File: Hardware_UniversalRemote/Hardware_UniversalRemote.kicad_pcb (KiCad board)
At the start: 2 copper layers, 140 x 140 mm, 58 parts, among them J1 USB_B_Micro, Q1 S8050, Q2 BSS138, Q3 S8050, Q4 S8050, Q5 S8050, Q6 S8050, Q7 S8050, SW1 SW_Push, SW2 SW_Push, SW3 SW_Push, U1 ESP32-WROOM-32U, U2 LM1117T-3.3, U3 HS0038B, U4 CH340C

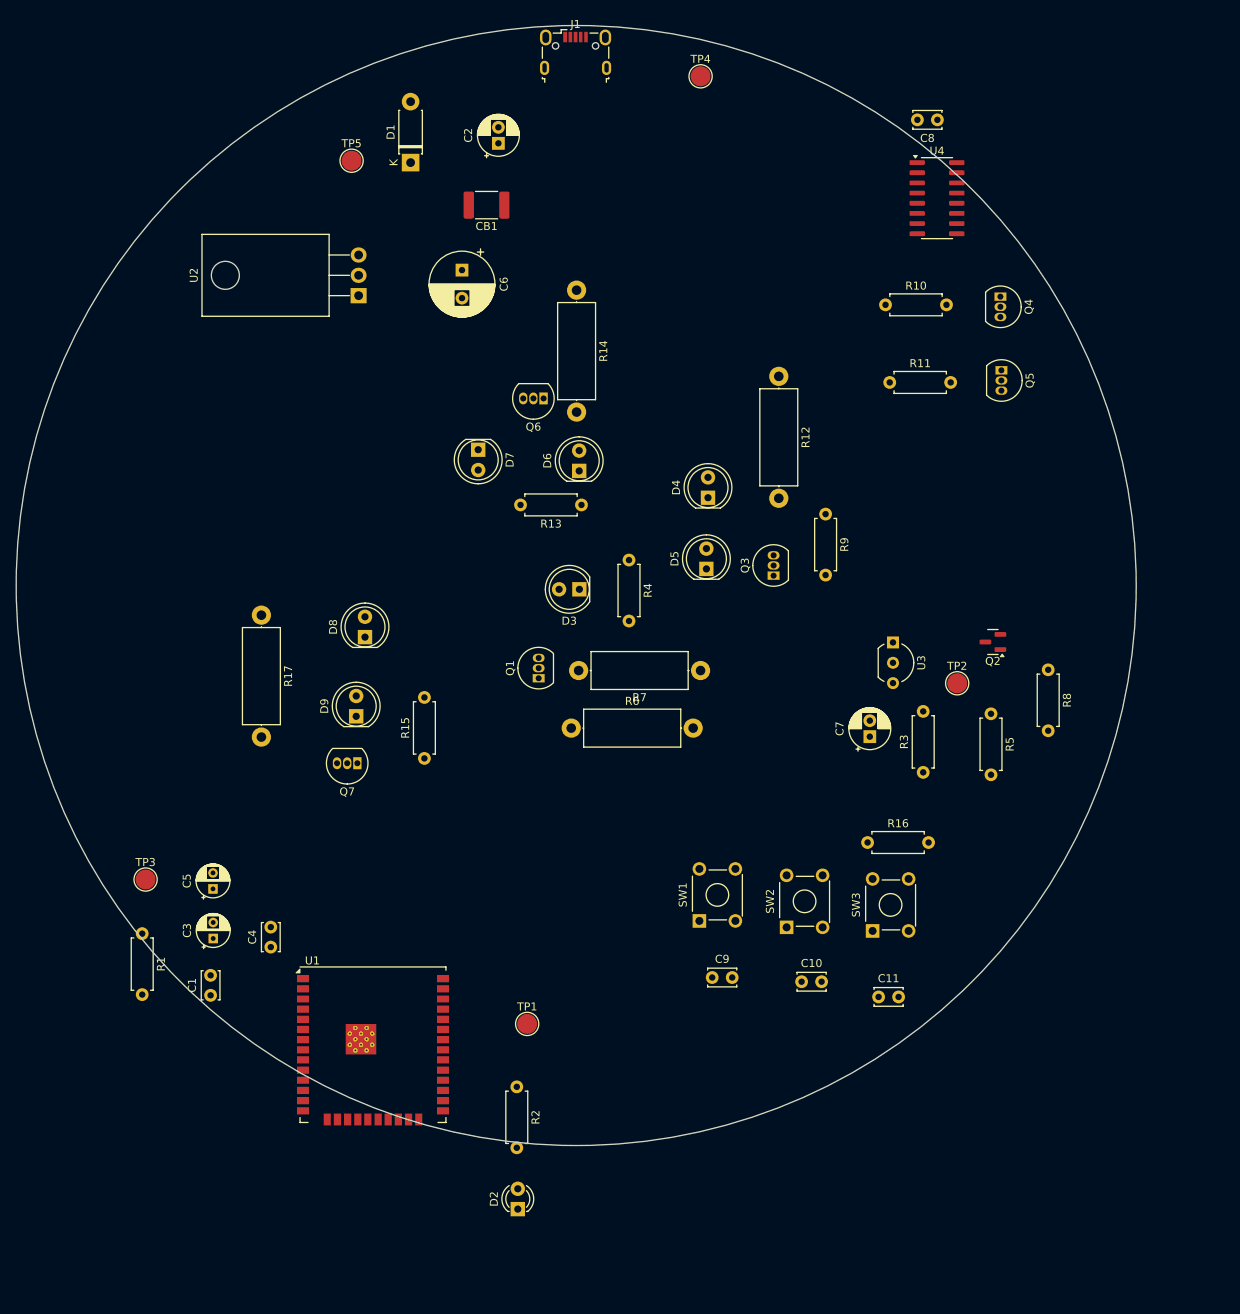
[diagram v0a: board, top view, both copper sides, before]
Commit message: add first pcb layout version
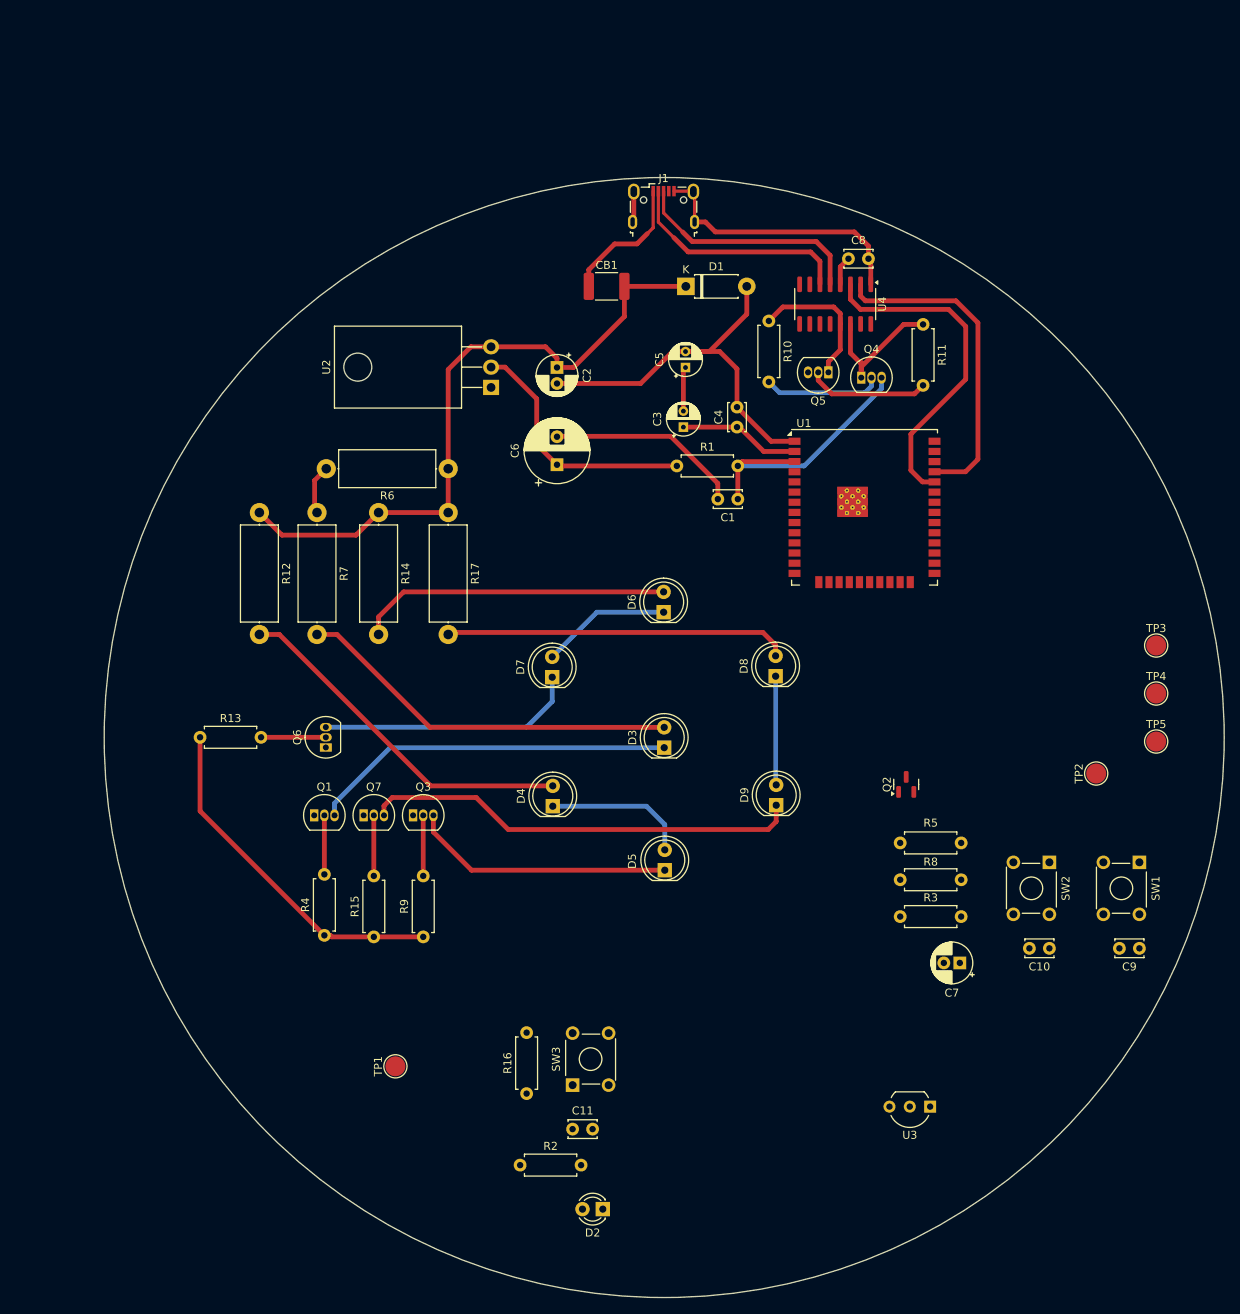
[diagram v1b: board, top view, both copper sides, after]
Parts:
- moved TP3 129.7 mm to (172.5, 107.5)
- moved TP5 124.0 mm to (172.5, 119.5)
- moved TP4 95.9 mm to (172.5, 113.5)
- moved U1 91.0 mm to (136.0, 90.2)
- moved C1 90.5 mm to (120.2, 89.2), turned to 180 degrees
- moved R1 88.8 mm to (112.6, 85.0), turned to 0 degrees
- moved C5 88.0 mm to (113.7, 72.8)
- moved C4 87.3 mm to (120.1, 80.2)
- moved C3 86.8 mm to (113.4, 80.2)
- moved R9 73.0 mm to (80.9, 143.9), turned to 90 degrees
- moved R12 67.1 mm to (60.4, 90.9)
- moved R4 60.4 mm to (68.5, 143.7), turned to 90 degrees
- moved U3 58.2 mm to (144.2, 165.1), turned to 180 degrees
- moved R13 55.8 mm to (53.0, 119.0), turned to 0 degrees
- moved SW1 55.5 mm to (170.4, 134.6), turned to -90 degrees
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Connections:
- C11 pad 1: /IO13 -> /IO16
- Q2 pad 2: /IO16 -> /IO13
- R16 pad 2: /IO13 -> /IO16
- R8 pad 1: /IO16 -> /IO13
- SW3 pad 1: /IO13 -> /IO16
- TP2 pad 1: /IO16 -> /IO13
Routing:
- net GND: track 0.00 -> 114.7 mm
- net +5V: track 0.00 -> 82.8 mm
- net Net-(D9-K): track 0.00 -> 54.8 mm
- net Net-(D3-A): track 0.00 -> 48.2 mm
- net Net-(D3-K): track 0.00 -> 45.6 mm
- net Net-(D4-A): track 0.00 -> 44.5 mm
- net /IO4: track 0.00 -> 43.6 mm
- net Net-(D8-A): track 0.00 -> 43.0 mm
- net /RXD0: track 0.00 -> 42.1 mm
- net /TXD0: track 0.00 -> 40.7 mm
- net Net-(D6-A): track 0.00 -> 39.1 mm
- net +3.3V: track 0.00 -> 35.3 mm
- net /EN: track 0.00 -> 34.8 mm
- net Net-(D5-K): track 0.00 -> 33.0 mm
- net Net-(D7-K): track 0.00 -> 32.7 mm
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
